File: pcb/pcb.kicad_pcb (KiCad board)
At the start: 2 copper layers, 10 parts

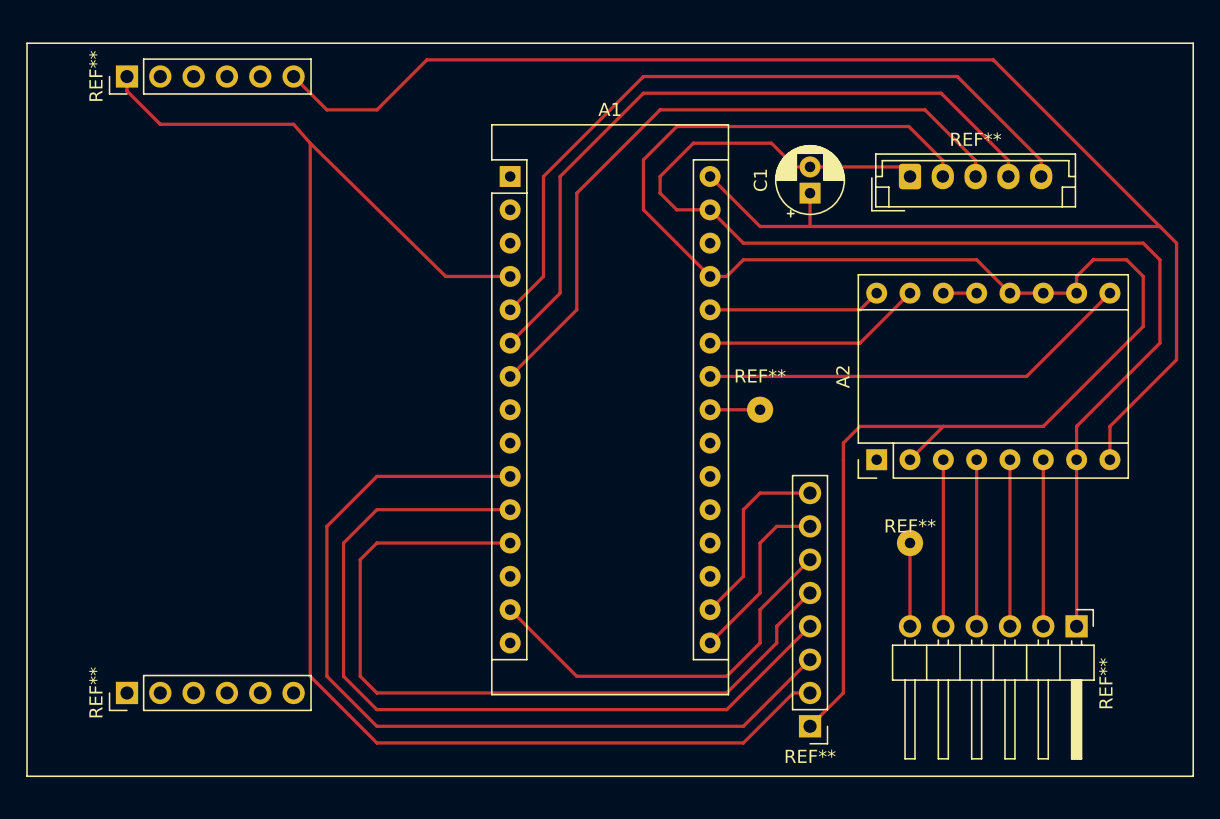
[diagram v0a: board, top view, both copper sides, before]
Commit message: update pcb
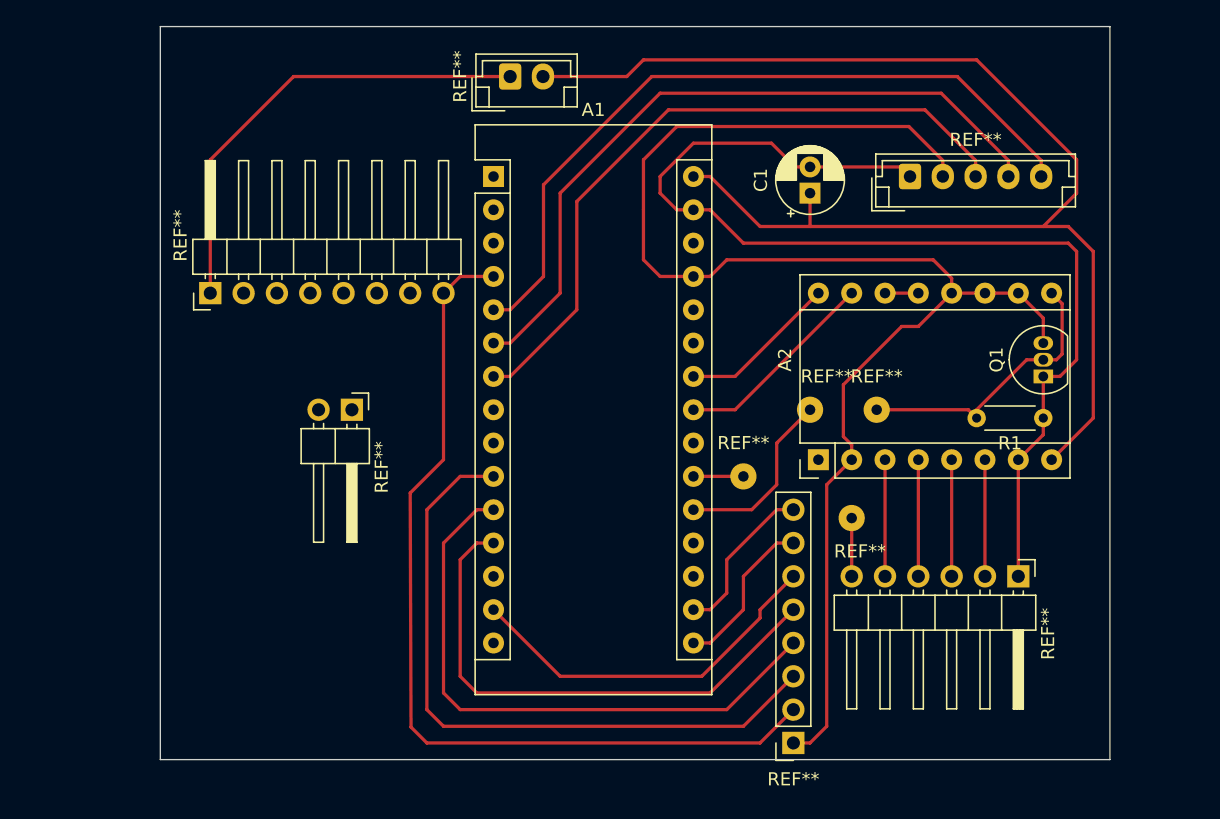
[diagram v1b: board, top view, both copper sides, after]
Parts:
- removed the REF** at (53.3, 90.2)
- removed the REF** at (53.3, 43.2)
- removed the REF** at (105.4, 92.7)
- added Q1: 2N3906, Package_TO_SOT_THT:TO-92_Inline, F.Cu at (123.2, 66.0)
- added R1: R, Resistor_THT:R_Axial_DIN0204_L3.6mm_D1.6mm_P5.08mm_Horizontal, F.Cu at (123.2, 69.2)
- added REF**: PinHeader_1x02_P2.54mm_Horizontal, Connector_PinHeader_2.54mm:PinHeader_1x02_P2.54mm_Horizontal, F.Cu at (70.5, 68.6)
- added REF**: PinSocket_1x08_P2.54mm_Vertical, Connector_PinSocket_2.54mm:PinSocket_1x08_P2.54mm_Vertical, F.Cu at (104.1, 94.0)
- added REF**: PinHeader_1x08_P2.54mm_Horizontal, Connector_PinHeader_2.54mm:PinHeader_1x08_P2.54mm_Horizontal, F.Cu at (59.7, 59.7)
- added REF**: JST_1x02, Connector_JST:JST_EH_B2B-EH-A_1x02_P2.50mm_Vertical, F.Cu at (82.5, 43.2)
- added REF**: pad, Connector_Wire:SolderWirePad_1x01_Drill0.8mm, F.Cu at (110.5, 68.6)
- added REF**: pad, Connector_Wire:SolderWirePad_1x01_Drill0.8mm, F.Cu at (105.4, 68.6)
- moved REF** 5.85 mm to (121.3, 81.3)
- moved REF** 5.24 mm to (100.3, 73.7)
- moved REF** 4.84 mm to (108.6, 76.8)
- moved A2 4.44 mm to (106.0, 72.4)
- moved A1 1.27 mm to (81.3, 50.8)
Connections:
- A2 pad 15: Net-(A1-Pad25) -> Net-(A1-Pad23)
- A2 pad 16: Net-(A2-Pad16) -> Net-(A1-Pad24)
- A2 pad 9: Net-(A1-Pad24) -> Net-(A1-Pad20)
- REF** pad 1: Net-(A1-Pad23) -> Net-(A1-Pad21)
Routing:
- net ardu_5v: track 130.7 -> 37.9 mm
- net ardu_5V: track 0.00 -> 72.9 mm
- net ardu_gnd2: track 118.6 -> 69.2 mm
- net Net-(A1-Pad20): track 0.00 -> 35.7 mm
- net (no net): track 0.00 -> 35.7 mm
- net ardu_vcc: track 132.7 -> 103.1 mm
- net Net-(A1-Pad24): track 33.1 -> 12.2 mm
- net tft_A0: track 59.6 -> 40.5 mm
- net tft_RES: track 63.2 -> 45.6 mm
- net Net-(A1-Pad25): track 16.8 -> 0.00 mm
- net tft_CS: track 67.5 -> 51.4 mm
- net Net-(A1-Pad26): track 13.2 -> 0.00 mm
- net Net-(A1-Pad23): track 3.81 -> 15.7 mm
- net ardu_gnd: track 93.2 -> 83.4 mm
- net stepper_2B: track 12.7 -> 8.89 mm
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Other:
- board outline added: 72.4 x 55.9 mm
